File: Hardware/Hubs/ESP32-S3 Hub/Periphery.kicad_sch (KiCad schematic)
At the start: 13 parts, among them SW1 Mitsumi R-667996, SW2 Mitsumi R-667996, SW3 DS04-254-2-04BK-SMT, U2 74HC595, U3 THVD1420DRLR

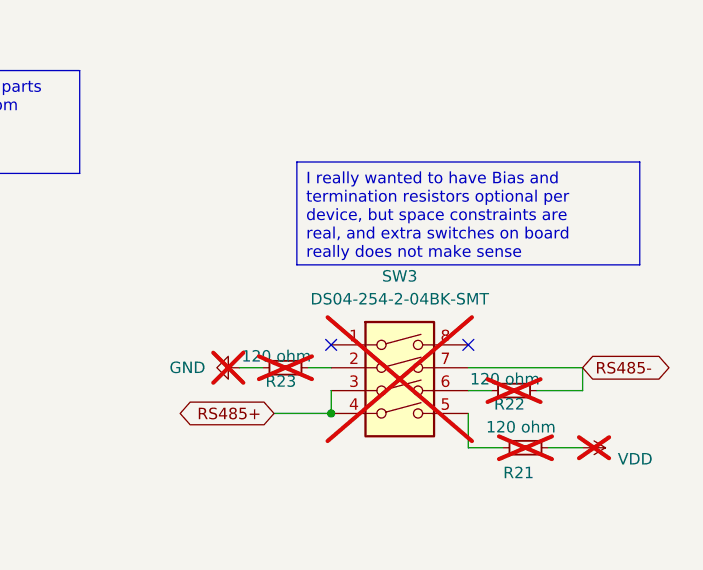
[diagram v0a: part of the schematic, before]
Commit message: Started Proto 2 again
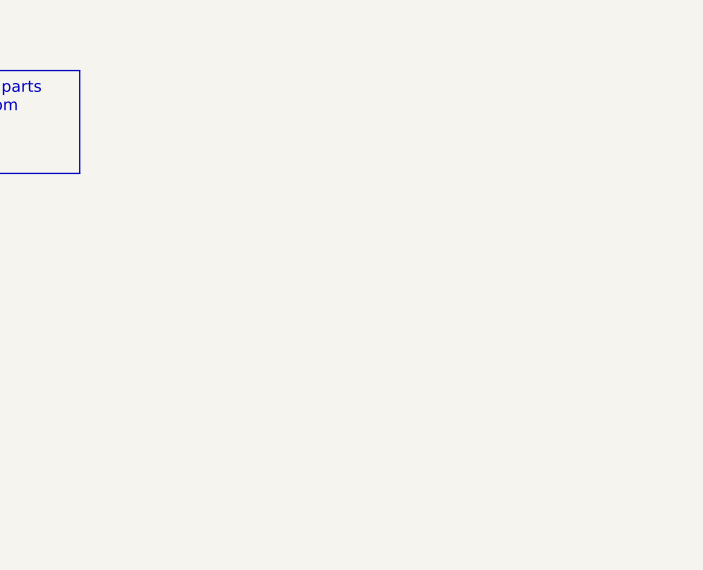
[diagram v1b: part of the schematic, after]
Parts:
- removed R21, R22, R23: 120 ohm, Resistor_SMD:R_0402_1005Metric, symbol Device:R_Small
- removed SW3: DS04-254-2-04BK-SMT, Button_Switch_SMD:SW_DIP_SPSTx04_Slide_Omron_A6S-410x_W8.9mm_P2.54mm, symbol Switch:SW_DIP_x04
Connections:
- no-connect marks 4 -> 2
